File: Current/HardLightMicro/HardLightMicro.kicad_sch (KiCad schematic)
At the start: 179 parts, among them J1 USB, K1 Keyswitch, K10 Keyswitch, K11 Keyswitch, K12 Keyswitch, K13 Keyswitch, K14 Keyswitch, K15 Keyswitch, K16 Keyswitch, K17 Keyswitch, K18 Keyswitch, K19 Keyswitch, K2 Keyswitch, K20 Keyswitch, K21 Keyswitch, K22 Keyswitch, K23 Keyswitch, K24 Keyswitch, K25 Keyswitch, K26 Keyswitch, K27 Keyswitch, K28 Keyswitch, K29 Keyswitch, K3 Keyswitch, K30 Keyswitch, K31 Keyswitch, K32 Keyswitch, K33 Keyswitch, K34 Keyswitch, K35 Keyswitch, K36 Keyswitch, K37 Keyswitch, K38 Keyswitch, K39 Keyswitch, K4 Keyswitch, K40 Keyswitch, K41 Keyswitch, K42 Keyswitch, K43 Keyswitch, K44 Keyswitch, K45 Keyswitch, K46 Keyswitch, K47 Keyswitch, K48 Keyswitch, K49 Keyswitch, K5 Keyswitch, K50 Keyswitch, K51 Keyswitch, K52 Keyswitch, K53 Keyswitch, K54 Keyswitch, K55 Keyswitch, K56 Keyswitch, K57 Keyswitch, K58 Keyswitch, K59 Keyswitch, K6 Keyswitch, K60 Keyswitch, K61 Keyswitch, K62 Keyswitch, K63 Keyswitch, K64 Keyswitch, K7 Keyswitch, K8 Keyswitch, K9 Keyswitch, U1 RP2040, U2 LDO-3.3, U3 W25Q128JVS, U4 USBLC6-2SC6, Y0 CSTCE12M0G55-R0

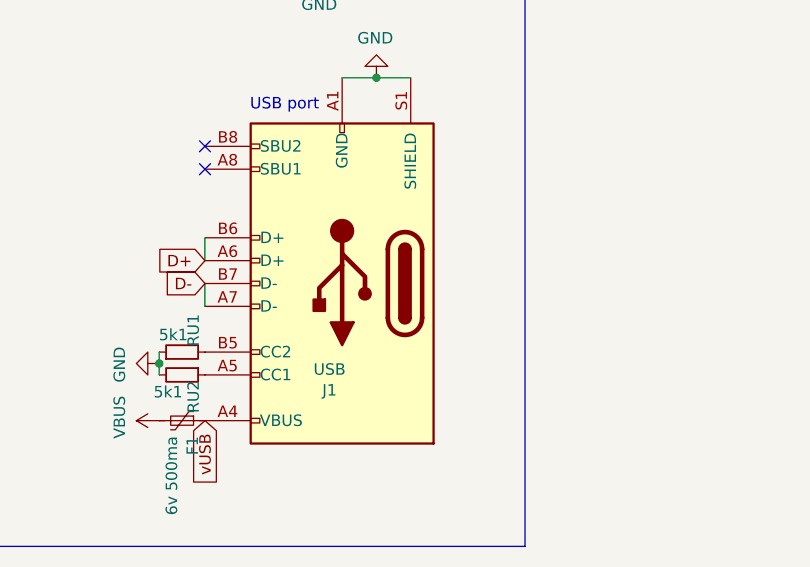
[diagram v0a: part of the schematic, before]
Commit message: Backup as of 2023.09.13
here we go kids quicksilver storm is now HARD LIGHT FINAL LET'S FUCKIN' GOOOOOOOOO
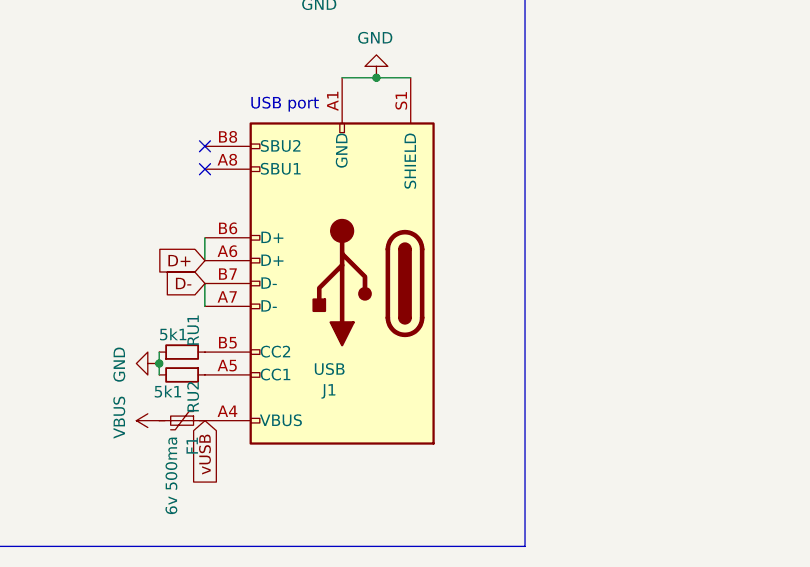
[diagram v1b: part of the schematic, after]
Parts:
- K1, K10, K11, K12, K13, K14, K15, K16, K17, K18, K19, K2, K20, K21, K22, K23, K24, K25, K26, K27, K28, K29, K3, K30, K31, K32, K33, K34, K35, K36, K37, K38, K39, K4, K40, K41, K42, K43, K44, K45, K46, K47, K48, K49, K5, K50, K51, K52, K53, K54, K55, K56, K57, K58, K59, K6, K60, K61, K62, K63, K64, K7, K8, K9: footprint EDI:GT-TC029B-H025-L1N -> EDI:SW_Micro_SKQG-Compat
